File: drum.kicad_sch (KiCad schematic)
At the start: 39 parts, among them J101 Cortex, J102 DX07S016JA3, SW101 SKSG, SW102 SKSG, U101 TPS78433QWDRBRQ1, U102 ATSAMD51J, Y101 32k768

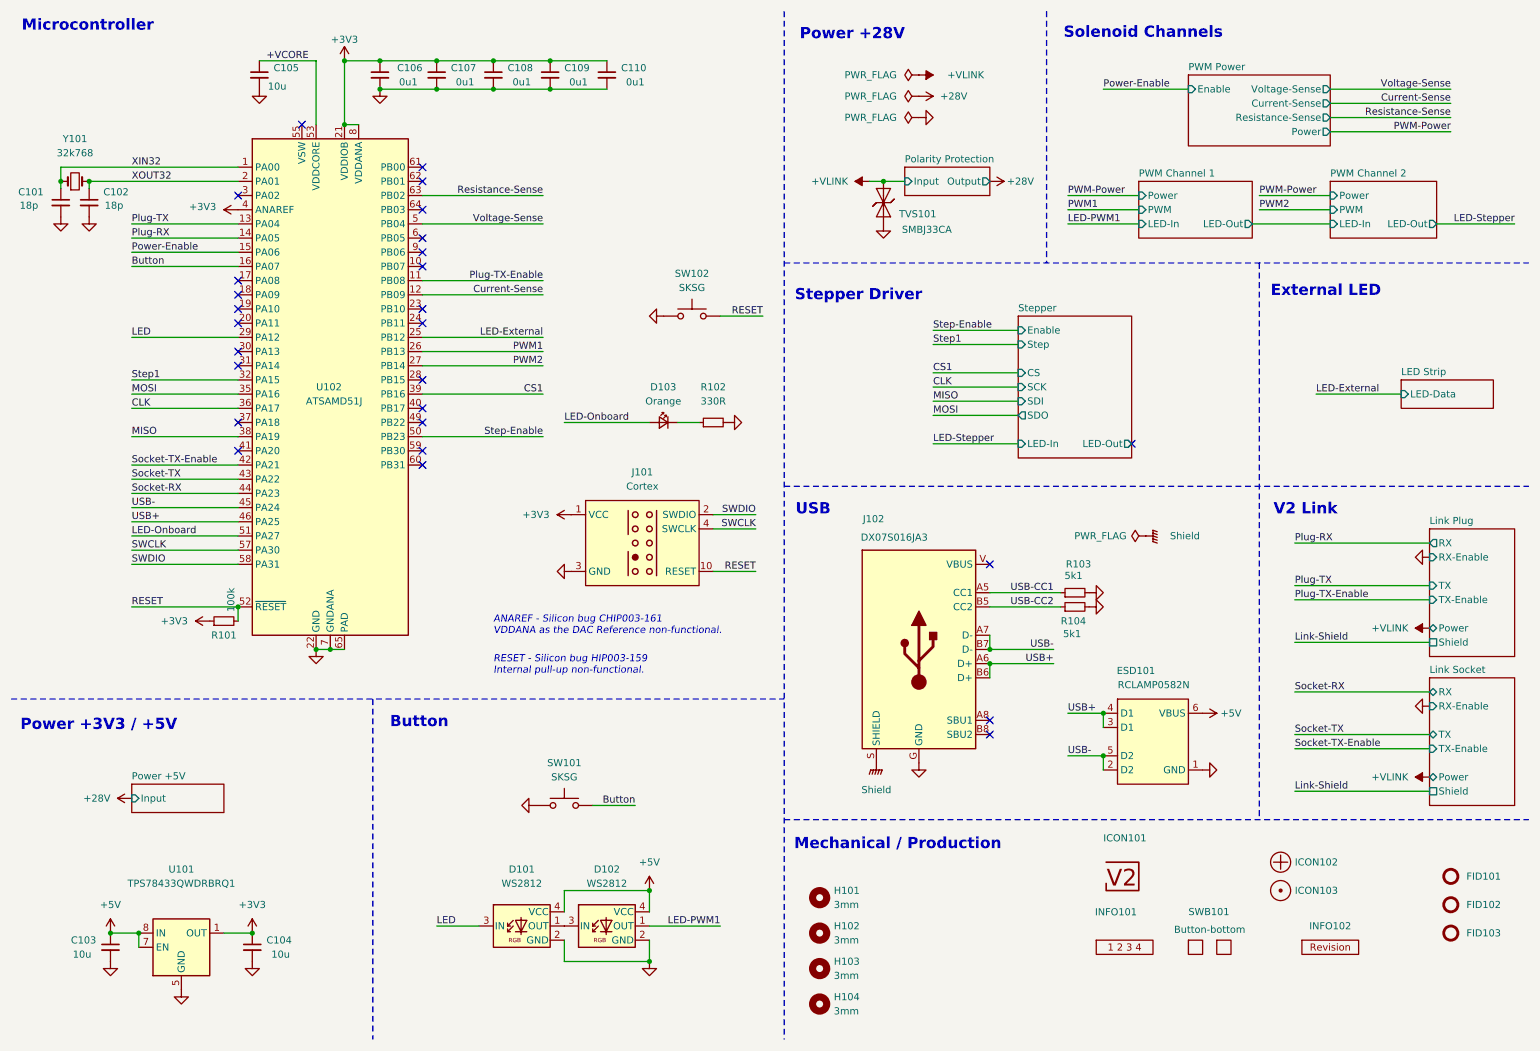
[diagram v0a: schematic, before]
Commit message: Refresh
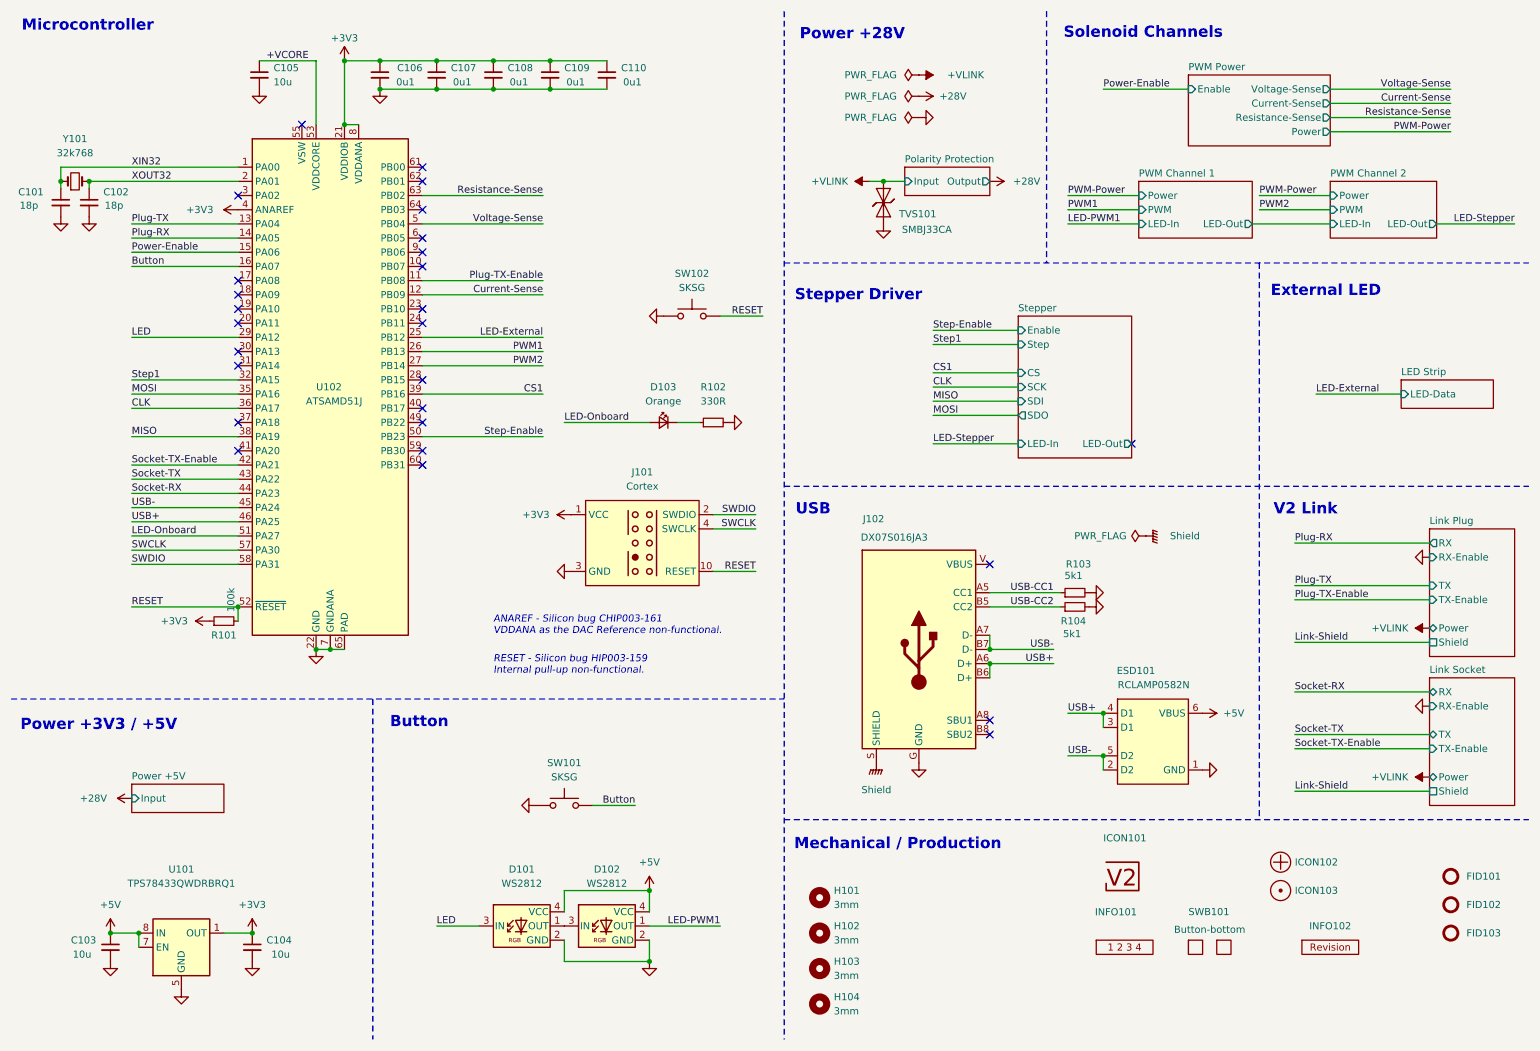
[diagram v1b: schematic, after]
